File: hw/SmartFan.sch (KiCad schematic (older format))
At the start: 68 parts, among them J1 Barrel_Jack, J2 JTAG_SWD, J7 FAN_CONN, Q1 MMBT2222A-7-F, Q10 2N3904, Q11 2N3904, Q12 2N3904, Q13 2N3904, Q14 2N3904, Q2 MMBT2222A-7-F, Q3 MMBT2222A-TP, Q4 MMBT2222A-TP, Q5 MMBT2222A-TP, Q6 MMBT2222A-7-F, Q7 MMBT2222A-7-F, Q8 MMBT2222A-7-F, Q9 2N3904, U1 L7805CV, U2 LTV-816S-TA1, U3 LTV-816S-TA1, U4 LTV-816S-TA1, U5 hackaBLE_0.3

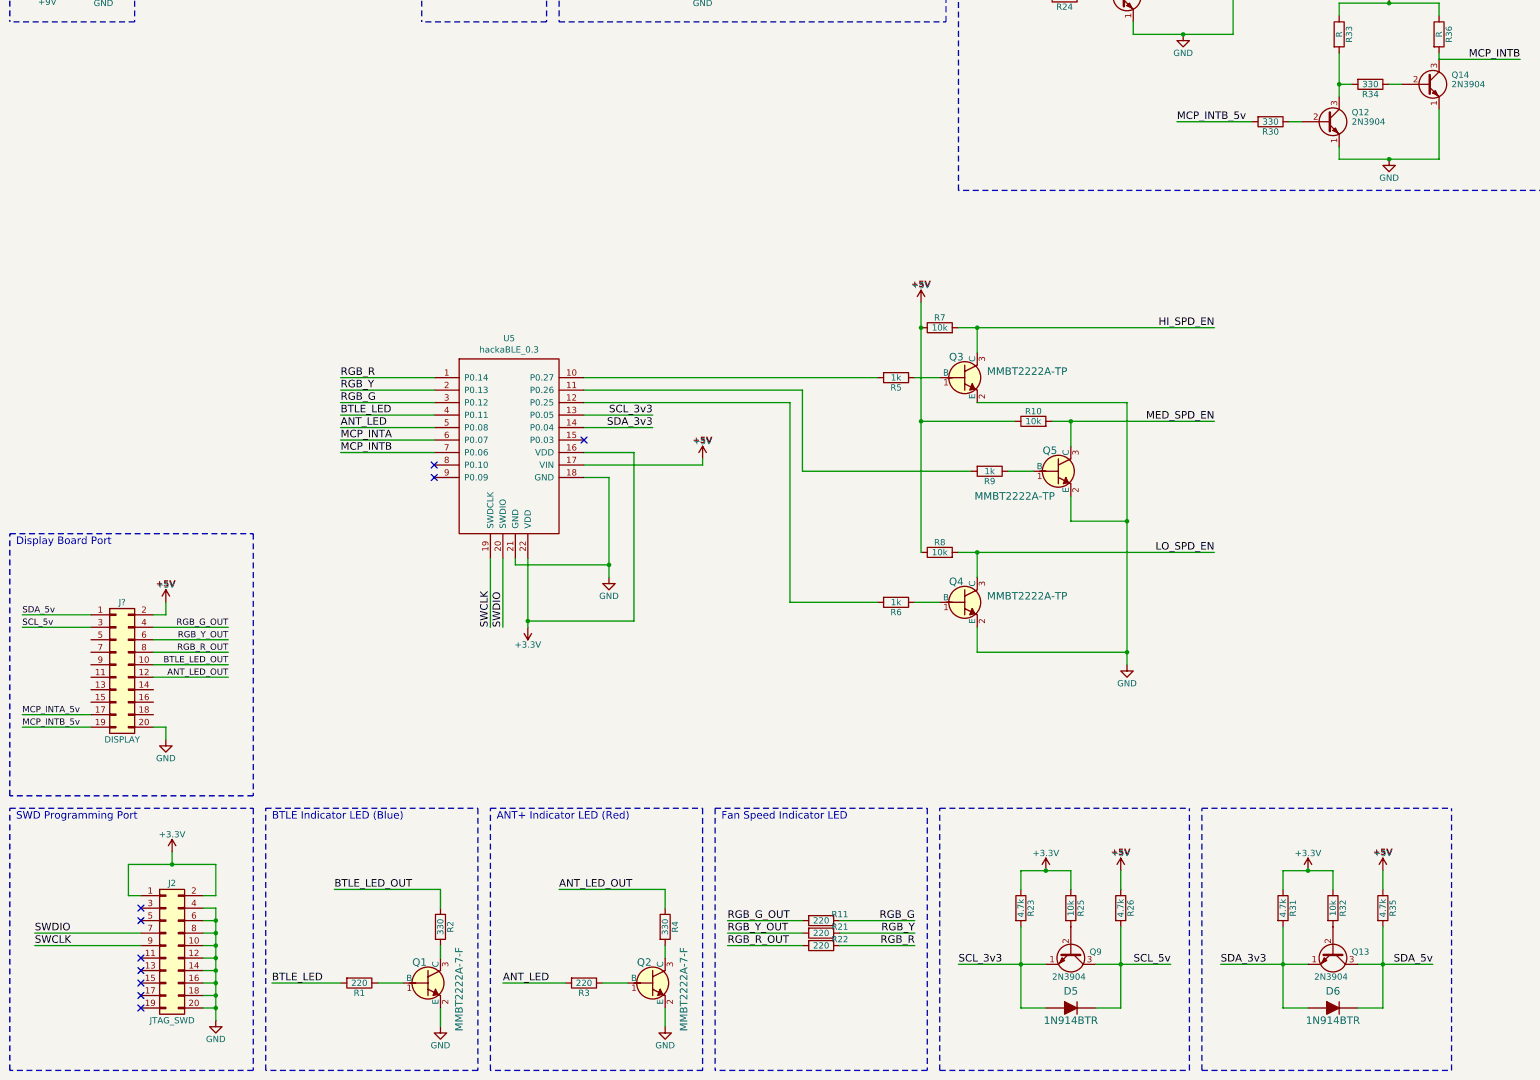
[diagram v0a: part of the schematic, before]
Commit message: mainboard updates
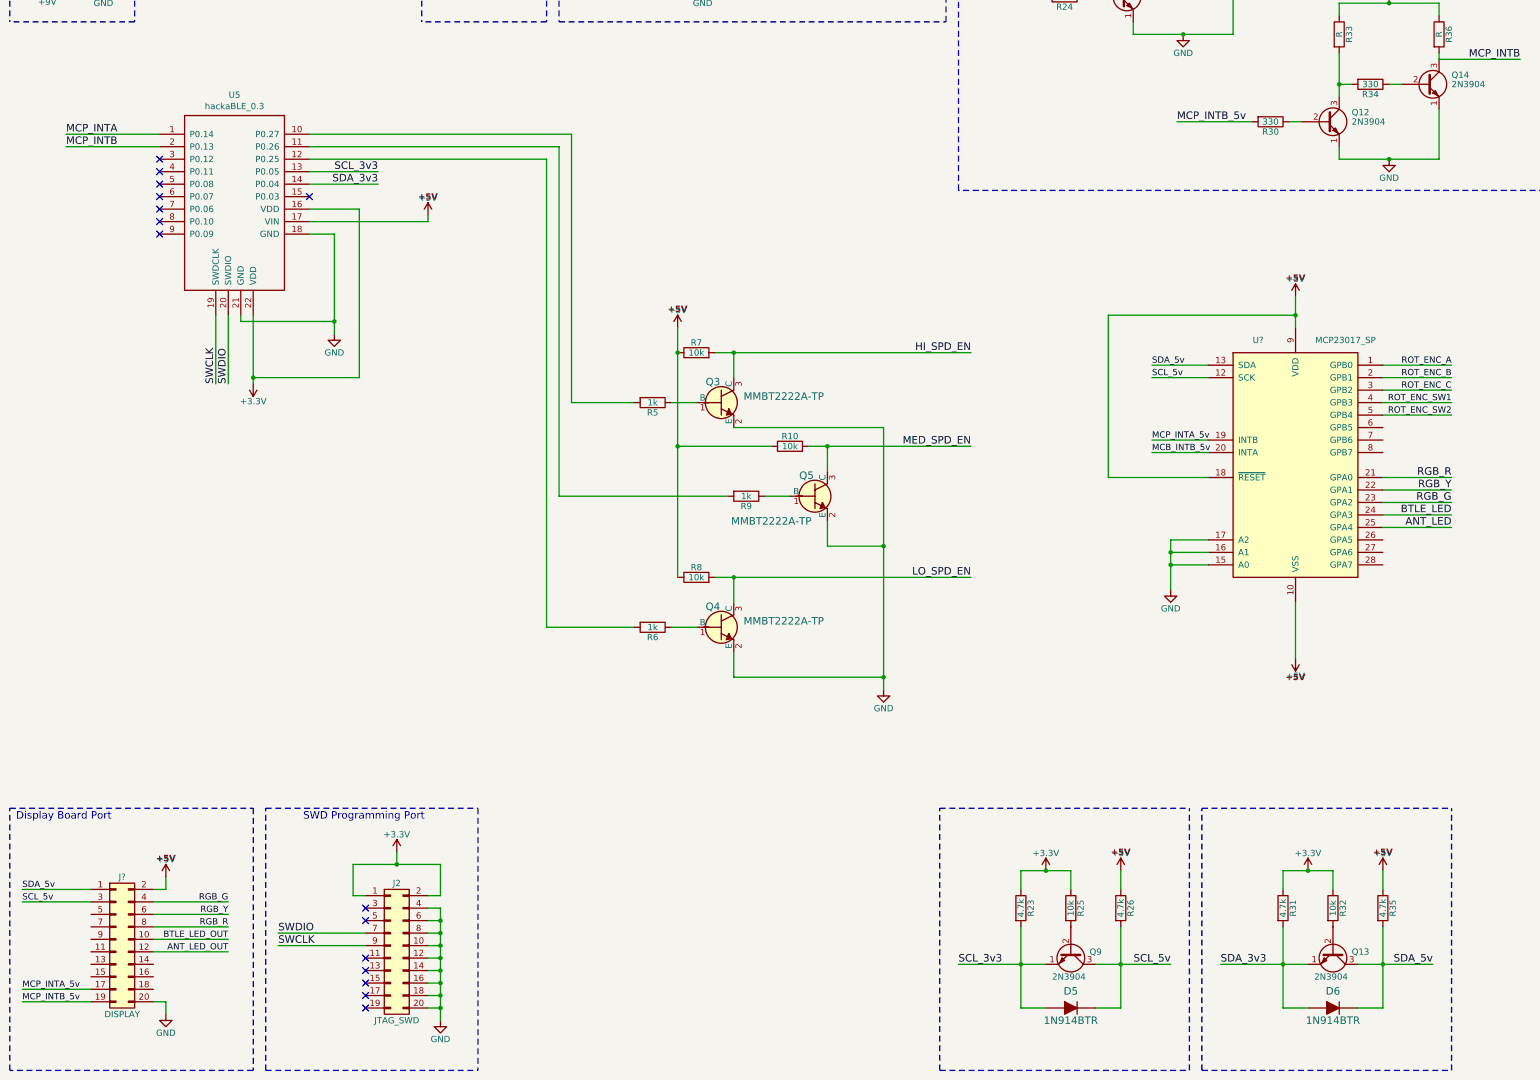
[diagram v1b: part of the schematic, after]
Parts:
- removed Q1, Q2: MMBT2222A-7-F, digikey-footprints:SOT-23-3, symbol SmartFan-rescue:MMBT2222A-7-F
- removed R1, R3: 220, Resistors_SMD:R_0805, symbol SmartFan-rescue:R
- removed R11, R21, R22: 220, symbol SmartFan-rescue:R
- removed R2, R4: 330, Resistors_SMD:R_0805, symbol SmartFan-rescue:R
- added U?: MCP23017_SP, Package_DIP:DIP-28_W7.62mm, symbol Interface_Expansion:MCP23017_SP
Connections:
- net RGB_G_OUT is gone; now on net RGB_G: J?.4 (Pin_4)
- net RGB_R_OUT is gone; now on net RGB_R: J?.8 (Pin_8)
- net RGB_Y_OUT is gone; now on net RGB_Y: J?.6 (Pin_6)
- net +5V: now also U?.10 (VSS), U?.18 (~RESET~), U?.9 (VDD)
- net ANT_LED: now also U?.25 (GPA4); no longer U5.5 (P0.08)
- net BTLE_LED: now also U?.24 (GPA3); no longer U5.4 (P0.11)
- net GND: now also U?.15 (A0), U?.16 (A1), U?.17 (A2)
- net MCP_INTA: now also U5.1 (P0.14); no longer U5.6 (P0.07)
- net MCP_INTA_5v: now also U?.19 (INTB)
- net MCP_INTB: now also U5.2 (P0.13); no longer U5.7 (P0.06)
- net RGB_G: now also U?.23 (GPA2); no longer U5.3 (P0.12)
- net RGB_R: now also U?.21 (GPA0); no longer U5.1 (P0.14)
- net RGB_Y: now also U?.22 (GPA1); no longer U5.2 (P0.13)
- net SCL_5v: now also U?.12 (SCK)
- net SDA_5v: now also U?.13 (SDA)
- new net MCB_INTB_5v: U?.20 (INTA)
- new net ROT_ENC_A: U?.1 (GPB0)
- new net ROT_ENC_B: U?.2 (GPB1)
- new net ROT_ENC_C: U?.3 (GPB2)
- new net ROT_ENC_SW1: U?.4 (GPB3)
- new net ROT_ENC_SW2: U?.5 (GPB4)
- no-connect marks 14 -> 19
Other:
- note removed: "ANT+ Indicator LED (Red)"
- note removed: "BTLE Indicator LED (Blue)"
- note removed: "Fan Speed Indicator LED"
- moved on the sheet: J2, J?, Q3, Q4, Q5, R10, R5, R6, R7, R8, R9, U5
